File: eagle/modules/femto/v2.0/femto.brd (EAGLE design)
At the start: 49.5 x 49.2 mm, 36 parts, among them IC1 MEGA8-AI, J1 RJ12RIGHTANGLE-I2C, J2 RJ12RIGHTANGLE-I2C, J3 RJ12RIGHTANGLE, J4 RJ12RIGHTANGLE, J5 RJ12RIGHTANGLE

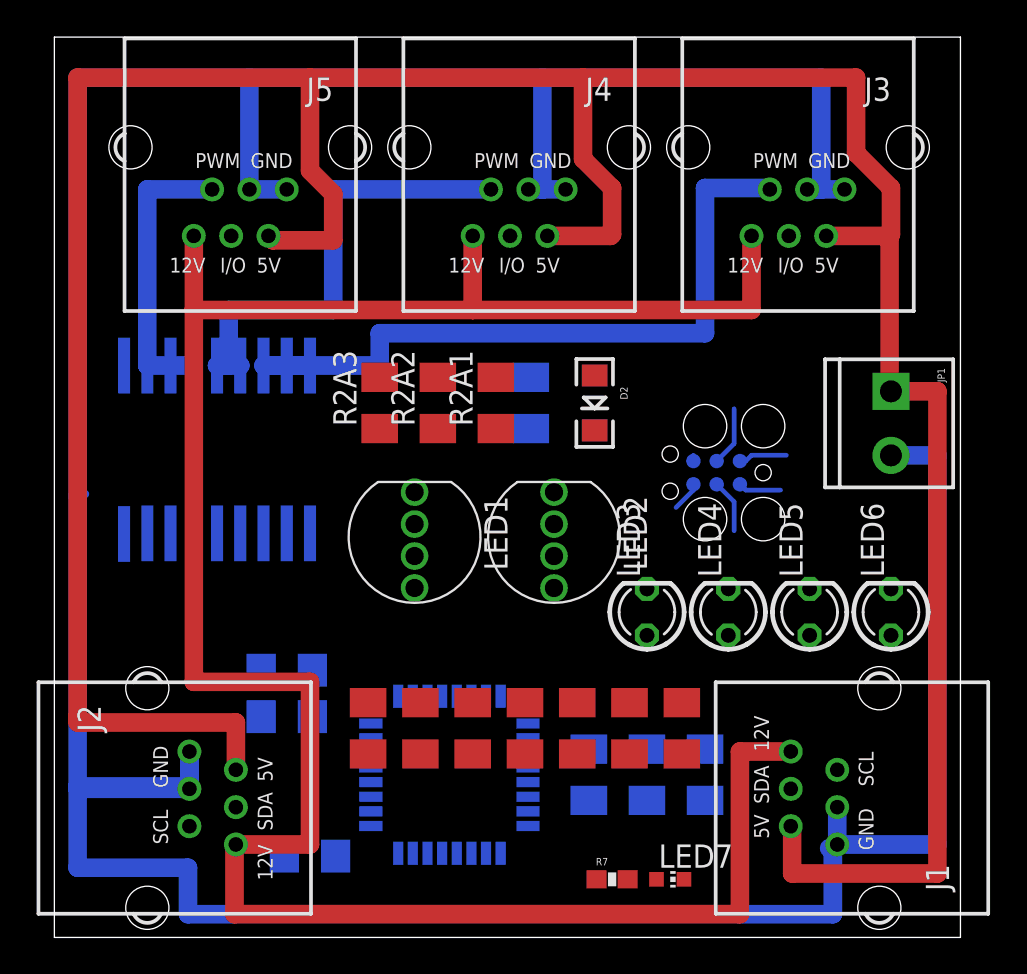
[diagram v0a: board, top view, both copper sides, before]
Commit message: Updaate
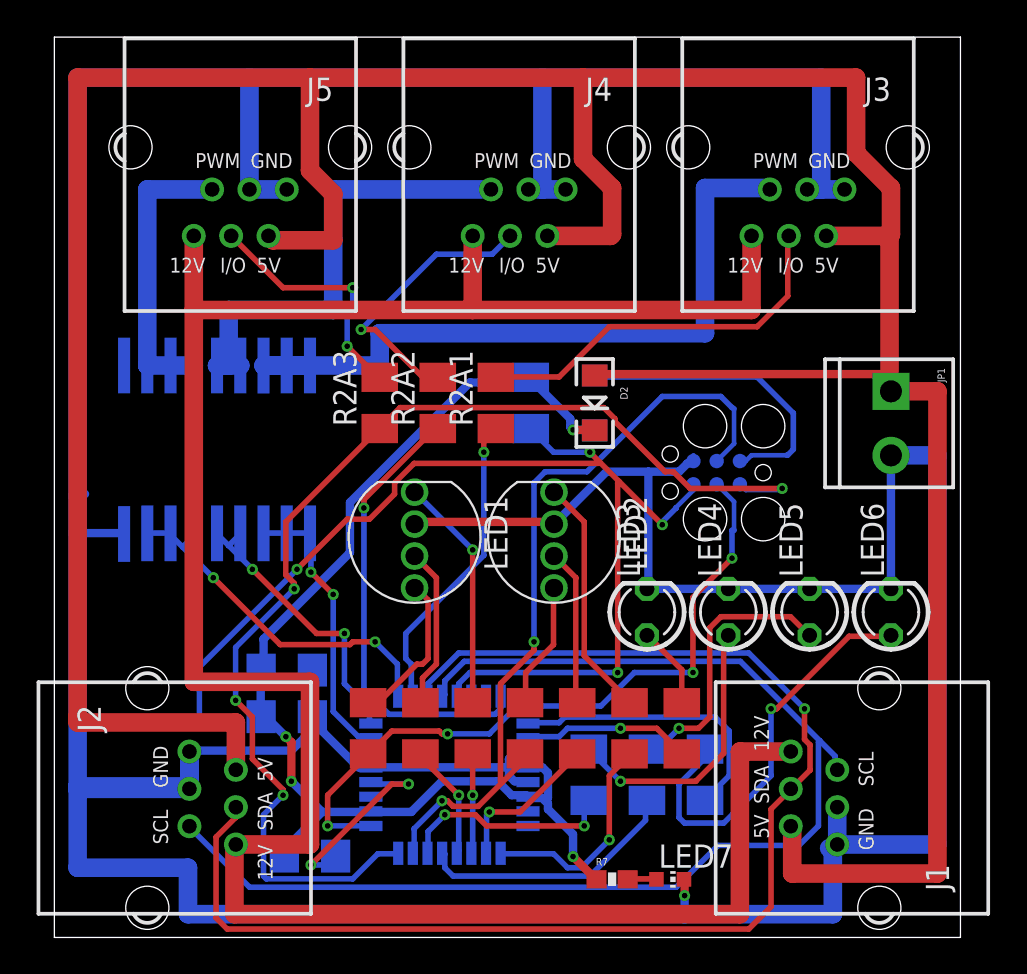
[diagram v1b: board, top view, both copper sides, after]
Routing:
- net GND: track 205.4 -> 279.8 mm, vias 0 -> 1
- net SDA: track 0.00 -> 72.6 mm, vias 0 -> 1
- net SCL: track 0.00 -> 67.5 mm
- net +5V: track 0.00 -> 64.4 mm, vias 0 -> 4
- net MISO: track 2.35 -> 64.5 mm, vias 0 -> 4
- net RESET: track 6.60 -> 67.2 mm, vias 0 -> 4
- net MOSI: track 3.25 -> 43.1 mm, vias 0 -> 2
- net SCK: track 2.93 -> 38.6 mm, vias 0 -> 4
- net D2: track 0.00 -> 24.9 mm, vias 0 -> 1
- net N$23: track 0.00 -> 22.5 mm, vias 0 -> 1
- net N$2: track 0.00 -> 21.1 mm
- net A2: track 0.00 -> 19.6 mm, vias 0 -> 2
- net 5V_B: track 176.3 -> 193.2 mm
- net A3: track 0.00 -> 16.8 mm, vias 0 -> 1
- net D3: track 0.00 -> 15.8 mm
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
